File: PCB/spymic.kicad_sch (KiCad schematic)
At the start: 0 parts

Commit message: c ommit
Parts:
- added C1, C2, C3, C8, C9: 10uF, symbol Device:C_Polarized
- added C4, C6, C7: 10uF, symbol Device:C
- added C5: 22uF, symbol Device:C
- added CN1: PJ-320D, easyeda2kicad:AUDIO-SMD_PJ-320D-1, symbol LCSC:PJ-320D
- added J1: 9V_Bat, symbol Connector:Conn_01x02_Pin
- added MK1: Piezo, symbol Device:Microphone_Crystal
- added R1: 50k, symbol Device:R
- added R2, R3: 1k, symbol Device:R
- added R4, R6: 470, symbol Device:R
- added R5: RK09K1130A5R, easyeda2kicad:RES-ADJ-TH_RK09K1130A5R, symbol LCSC:RK09K1130A5R
- added U1: GS8331-TR, easyeda2kicad:SOT-23-5_L3.0-W1.7-P0.95-LS2.8-BL, symbol LCSC:GS8331-TR
- added U2: ICL7660M/TR, easyeda2kicad:SOP-8_L4.9-W3.9-P1.27-LS6.0-BL, symbol LCSC:ICL7660M_TR
- added U3: XC62KN3302PR-G, easyeda2kicad:SOT-89-3_L4.5-W2.5-P1.50-LS4.2-BR, symbol LCSC:XC62KN3302PR-G
- added U4: XC6206P332MR, easyeda2kicad:SOT-23-3_L2.9-W1.6-P1.90-LS2.8-BR, symbol LCSC:XC6206P332MR
- added U5: K7805M-1000R3_C41361052, easyeda2kicad:PWRM-TH_DEXU_K780XM-1000R3, symbol LCSC:K7805M-1000R3_C41361052
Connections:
- new net: CN1.4, R6.2
- new net: R2.1, R3.1, U1.4 (INA-)
- new net: MK1.2 (+), R1.1, U1.3 (INA+)
- new net: CN1.3, R4.2
- new net: R3.2, R5.3
- new net: C1.1, U2.2 (CAP+)
- new net: C1.2, U2.4 (CAP–)
- new net: C4.1, J1.9V+ (Pin_1), U5.1 (VIN)
- new net 3V3+: C6.1, U1.2 (V-), U4.2 (Vout)
- new net 3V3-: C8.2, U1.5 (V+), U3.3 (-VIN)
- new net 5V+: C2.1, C5.1, C7.1, U2.8 (V+), U4.3 (Vin), U5.3 (VOUT)
- new net 5V-: C3.2, C9.2, U2.5 (VOUT), U3.1 (-VOUT)
- new net GND: C2.2, C3.1, C4.2, C5.2, C6.2, C7.2, C8.1, C9.1, CN1.1, J1.9V- (Pin_2), MK1.1 (-), R1.2, R2.2, U2.3 (GND), U2.6 (LV), U3.2 (VSS), U4.1 (GND), U5.2 (GND)
- new net SIG: R5.2, U1.1 (OUTA)
- no-connect marks 0 -> 4

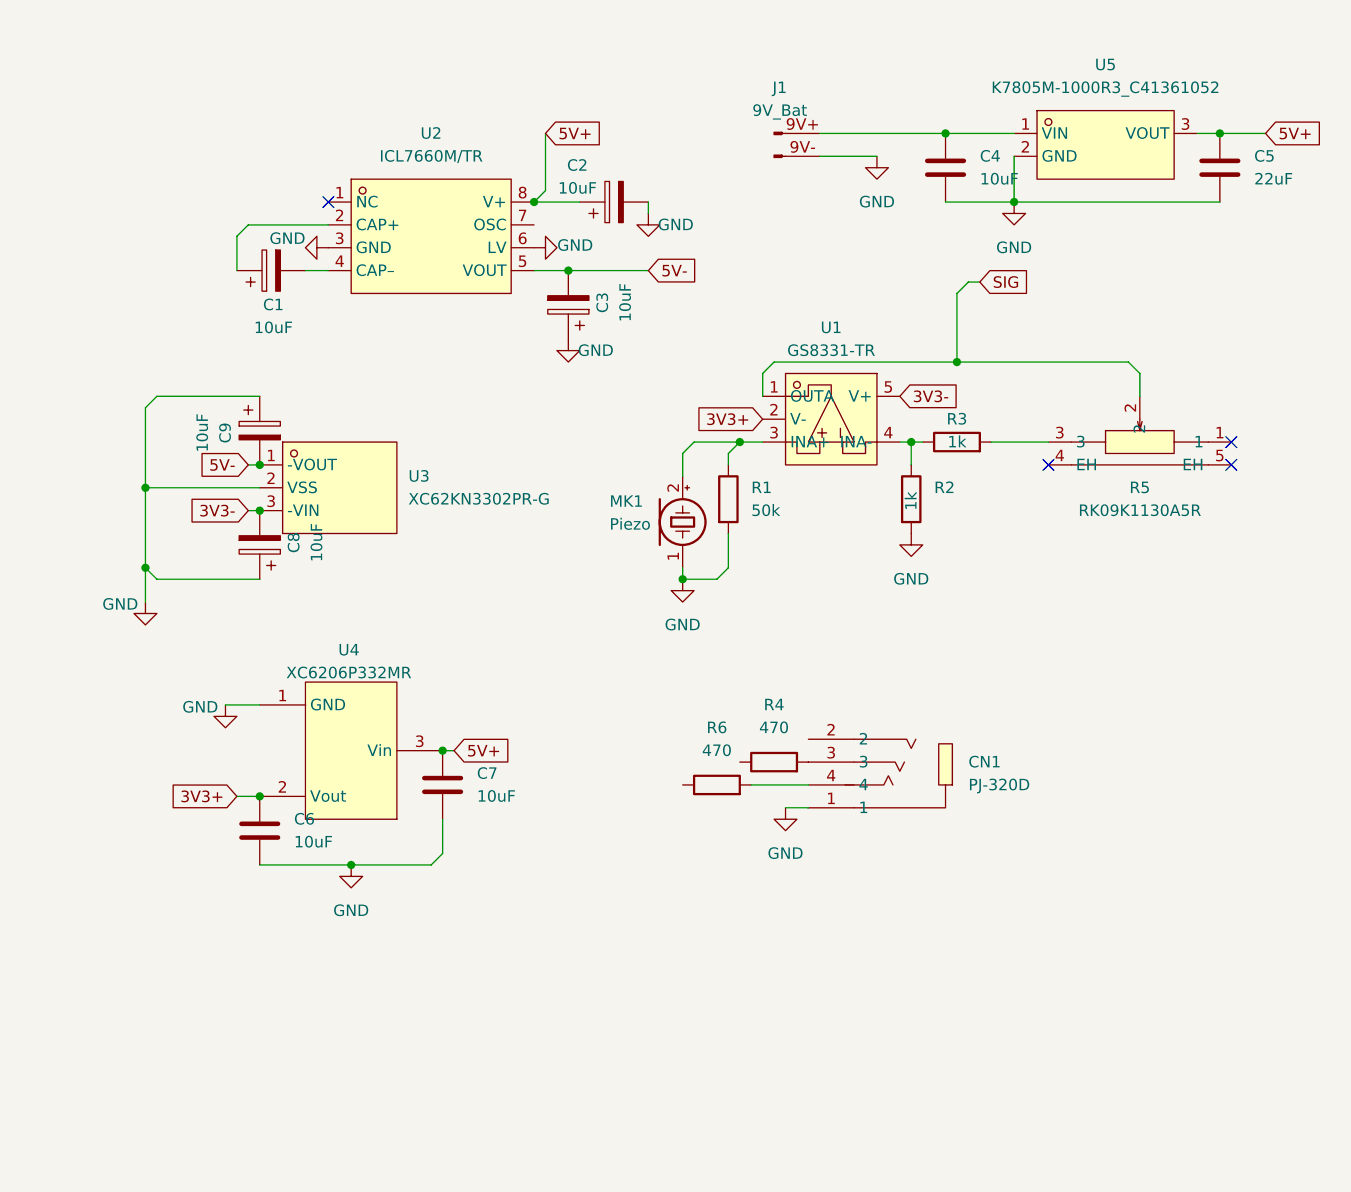
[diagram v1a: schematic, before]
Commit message: huge journal backlog
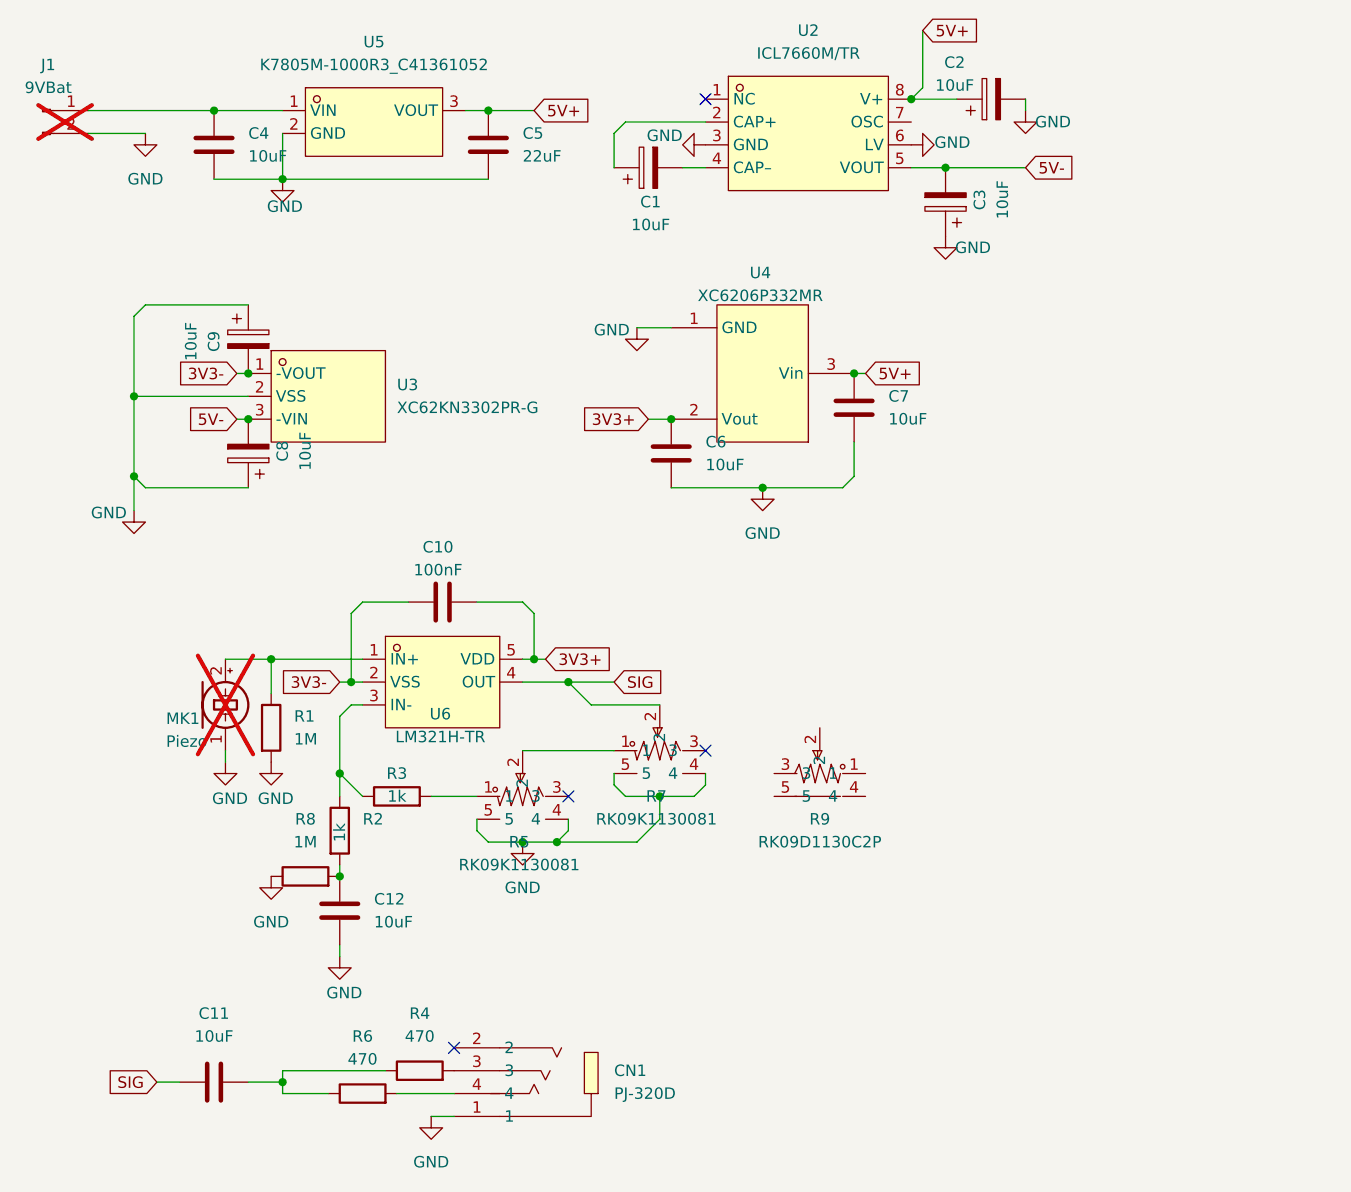
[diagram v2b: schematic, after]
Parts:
- removed R5: RK09K1130A5R, easyeda2kicad:RES-ADJ-TH_RK09K1130A5R, symbol LCSC:RK09K1130A5R
- removed U1: GS8331-TR, easyeda2kicad:SOT-23-5_L3.0-W1.7-P0.95-LS2.8-BL, symbol LCSC:GS8331-TR
- added C10: 100nF, Capacitor_SMD:C_0603_1608Metric_Pad1.08x0.95mm_HandSolder, symbol Device:C
- added C11, C12: 10uF, Capacitor_SMD:C_0603_1608Metric_Pad1.08x0.95mm_HandSolder, symbol Device:C
- added R5, R7: RK09K1130081, easyeda2kicad:RES-TH_RK09K1130AAU, symbol LCSC:RK09K1130081
- added R8: 1M, Resistor_SMD:R_1206_3216Metric_Pad1.30x1.75mm_HandSolder, symbol Device:R
- added R9: RK09D1130C2P, easyeda2kicad:RES-TH_RK09D1130C2P, symbol LCSC:RK09D1130C2P
- added U6: LM321H-TR, easyeda2kicad:SOT-23-5_L2.9-W1.6-P0.95-LS2.8-BL, symbol LCSC:LM321H-TR
- C1, C2, C3, C8, C9: footprint (none) -> Capacitor_SMD:CP_Elec_4x5.4; LCSC Part (none) -> C72485
- C4, C6, C7: footprint (none) -> Capacitor_SMD:C_0603_1608Metric_Pad1.08x0.95mm_HandSolder; LCSC Part (none) -> C1691
- C5: footprint (none) -> Capacitor_SMD:C_0603_1608Metric_Pad1.08x0.95mm_HandSolder; LCSC Part (none) -> C59461
- J1: value 9V_Bat -> 9VBat; footprint (none) -> Connector_Wire:SolderWire-0.25sqmm_1x02_P4.5mm_D0.65mm_OD2mm_Relief; now not fitted
- MK1: footprint (none) -> Connector_Wire:SolderWire-0.25sqmm_1x02_P4.5mm_D0.65mm_OD2mm_Relief; now not fitted
- R1: value 50k -> 1M; footprint (none) -> Resistor_SMD:R_1206_3216Metric_Pad1.30x1.75mm_HandSolder; LCSC Part (none) -> C17927
- R2, R3: footprint (none) -> Resistor_SMD:R_0603_1608Metric_Pad0.98x0.95mm_HandSolder; LCSC Part (none) -> C2907002
- R4, R6: footprint (none) -> Resistor_SMD:R_0603_1608Metric_Pad0.98x0.95mm_HandSolder; LCSC Part (none) -> C23179
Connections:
- net 3V3+: now also C10.2, U6.5 (VDD)
- net 3V3-: now also C9.2, U3.1 (-VOUT), C10.1, U6.2 (VSS); no longer C8.2, U3.3 (-VIN)
- net 5V-: now also C8.2, U3.3 (-VIN); no longer C9.2, U3.1 (-VOUT)
- net GND: now also J1.2 (Pin_2), C12.2, R5.4, R5.5, R7.4, R7.5, R8.1; no longer J1.9V- (Pin_2), R2.2
- net SIG: now also C11.1, R7.2, U6.4 (OUT)
- net at R6.1: now also R4.1, C11.2
- net at R2.1, R3.1: now also U6.3 (IN-)
- net at MK1.2 (+), R1.1: now also U6.1 (IN+)
- net at R3.2: now also R5.1
- net at C4.1, U5.1 (VIN): now also J1.1 (Pin_1); no longer J1.9V+ (Pin_1)
- new net: C12.1, R2.2, R8.2
- new net: R5.2, R7.1
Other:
- moved on the sheet: C1, C2, C3, C4, C5, C6, C7, C8, C9, CN1, R1, R2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
